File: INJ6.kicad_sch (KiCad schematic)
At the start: 9 parts, among them U10 VNLD5160TR-E, U11 VNLD5160TR-E, U9 VNLD5160TR-E

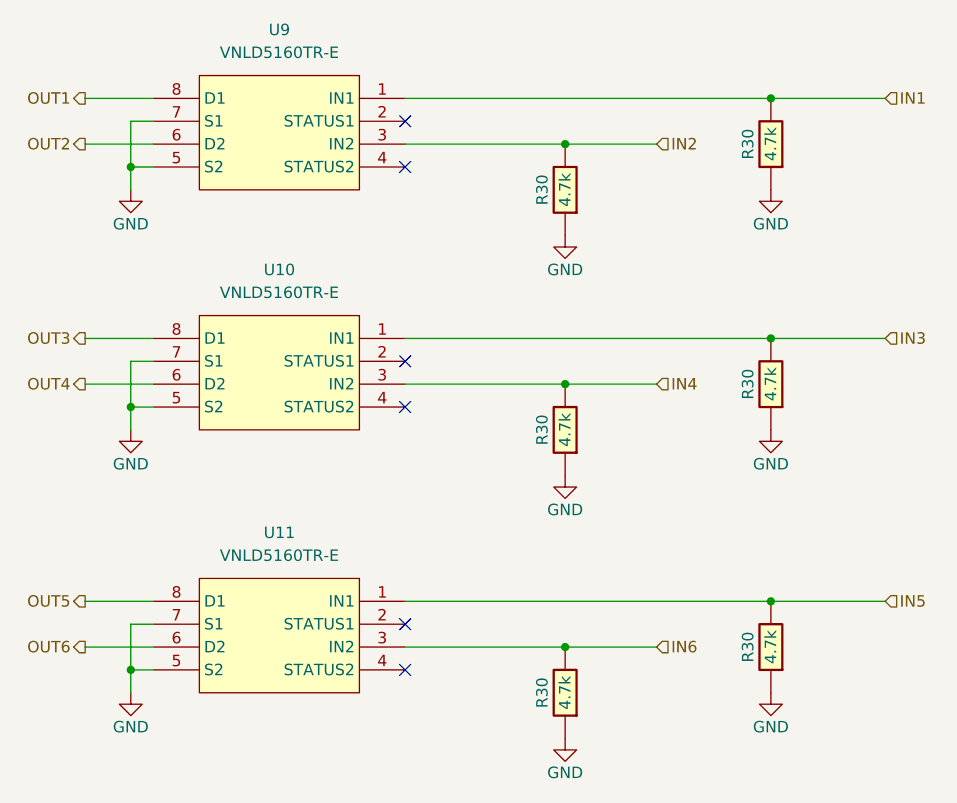
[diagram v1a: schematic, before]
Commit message: test
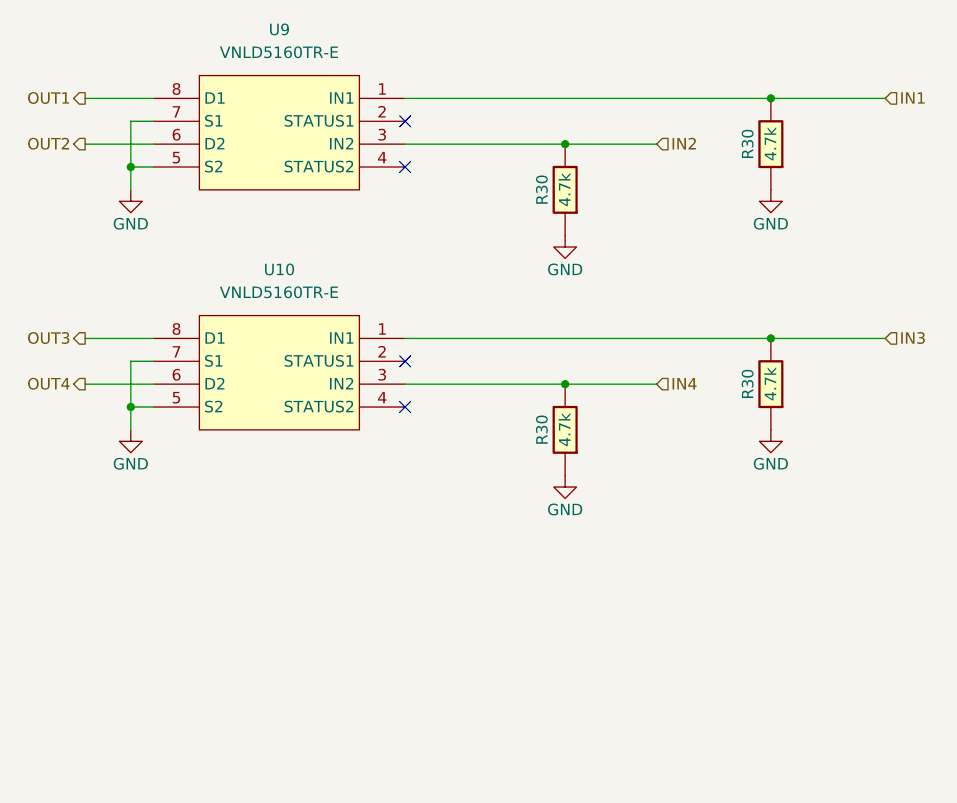
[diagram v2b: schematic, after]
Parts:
- removed R30 (x2): 4.7k, hellen-one-common:R0603, symbol hellen-one-common:Res
- removed U11: VNLD5160TR-E, Package_SO:SOIC-8_3.9x4.9mm_P1.27mm, symbol chips:VNLD5160
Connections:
- no-connect marks 6 -> 4

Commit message: reset
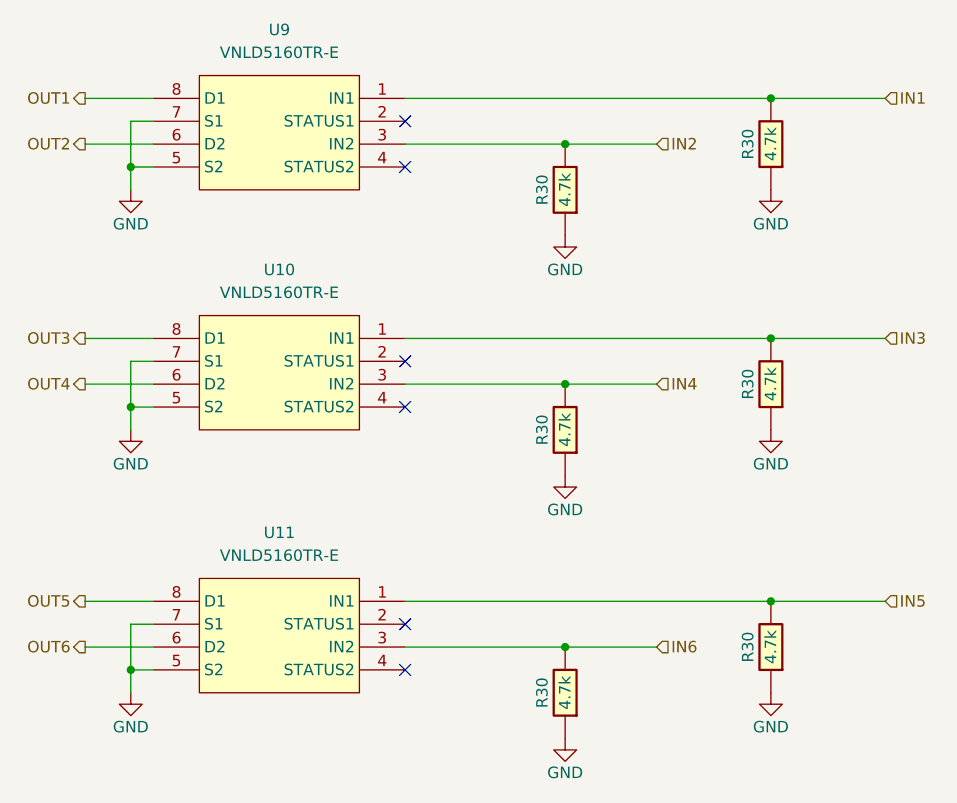
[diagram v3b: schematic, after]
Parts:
- added R30 (x2): 4.7k, hellen-one-common:R0603, symbol hellen-one-common:Res
- added U11: VNLD5160TR-E, Package_SO:SOIC-8_3.9x4.9mm_P1.27mm, symbol chips:VNLD5160
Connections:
- net GND: now also R30.1, R30.1, U11.5 (S2), U11.7 (S1)
- new net IN5: R30.2, U11.1 (IN1)
- new net IN6: R30.2, U11.3 (IN2)
- new net OUT5: U11.8 (D1)
- new net OUT6: U11.6 (D2)
- no-connect marks 4 -> 6
